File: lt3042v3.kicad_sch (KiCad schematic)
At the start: 8 parts, among them U4 LT3094MPDD-PBF

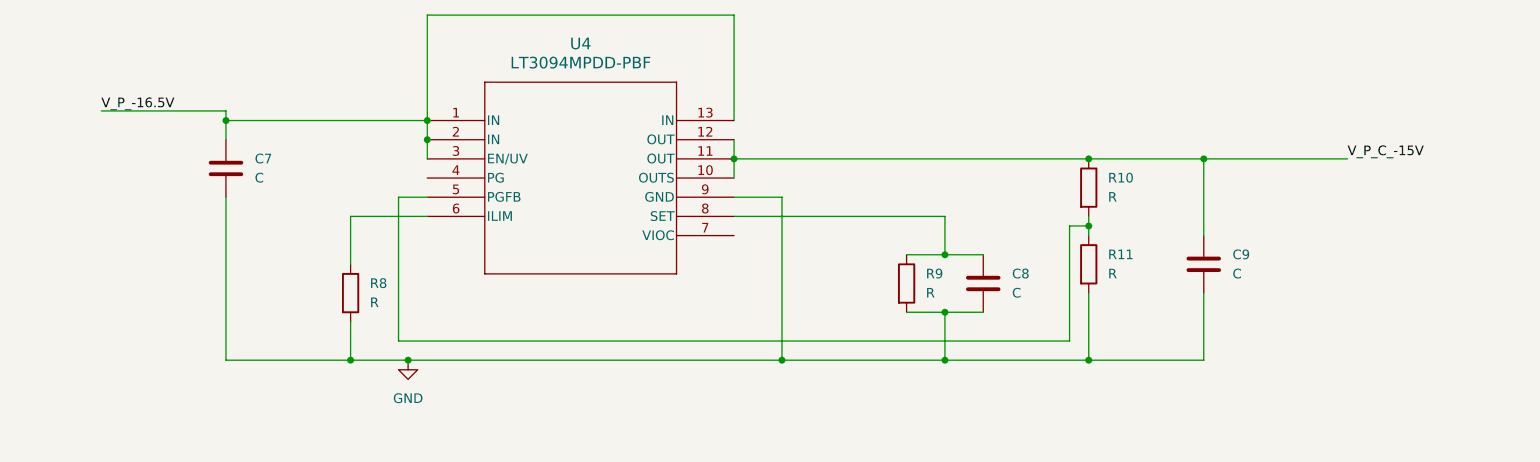
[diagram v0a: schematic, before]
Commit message: main
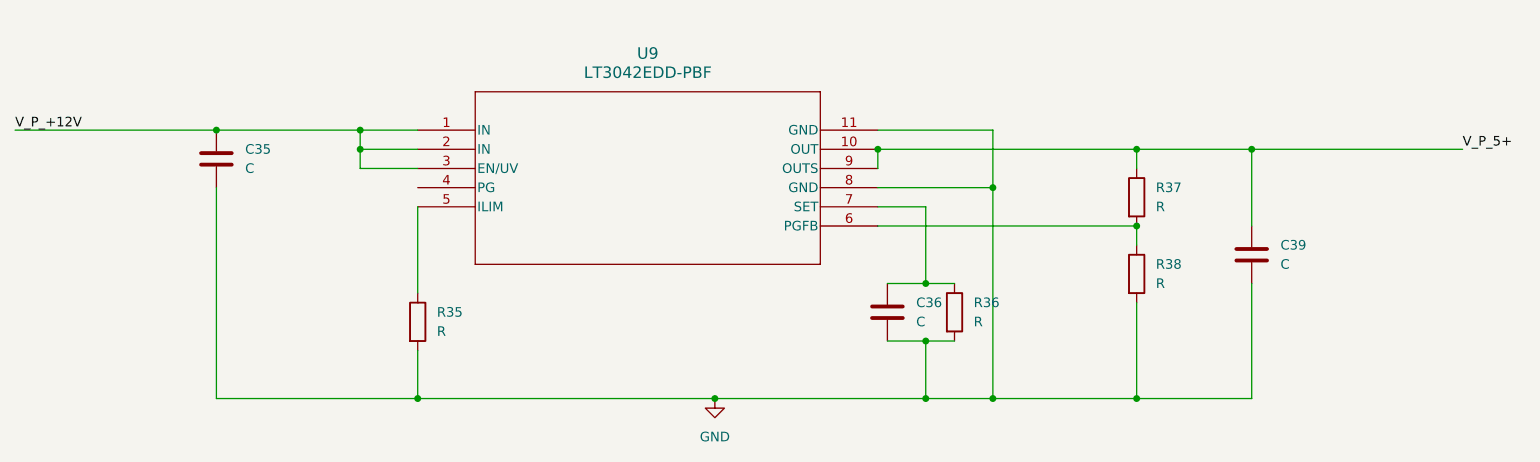
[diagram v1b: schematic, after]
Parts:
- removed C7, C8, C9: C, symbol Device:C
- removed R10, R11, R8, R9: R, symbol Device:R
- removed U4: LT3094MPDD-PBF, DD_05-08-1725_ADI, symbol 2026-06-29_19-42-13:LT3094MPDD-PBF
- added C35, C36, C39: C, symbol Device:C
- added R35, R36, R37, R38: R, symbol Device:R
- added U9: LT3042EDD-PBF, DFN-10_DD_LIT, symbol 2026-06-29_19-42-44:LT3042EDD-PBF
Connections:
- net GND: now also C35.2, C36.2, C39.2, R35.2, R36.2, R38.2, U9.11 (GND), U9.8 (GND)
- new net: R35.1, U9.5 (ILIM)
- new net: R37.2, R38.1, U9.6 (PGFB)
- new net: C36.1, R36.1, U9.7 (SET)
- new net V_P_+12V: C35.1, U9.1 (IN), U9.2 (IN), U9.3 (EN/UV)
- new net V_P_5+: C39.1, R37.1, U9.10 (OUT), U9.9 (OUTS)
